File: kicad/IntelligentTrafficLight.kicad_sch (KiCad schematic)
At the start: 62 parts, among them J1 Conn_01x03_Pin, J2 Conn_01x10_Socket, J3 USB-C Receptacle, J4 Conn_01x07_Socket, J5 Conn_01x07_Socket, SW1 Pushbutton, SW2 Pushbutton, U1 ESP32-C3-MINI-1-H4X, U2 PCA9685PW, U3 TLV76133DCY, U4 MAX40200AUK

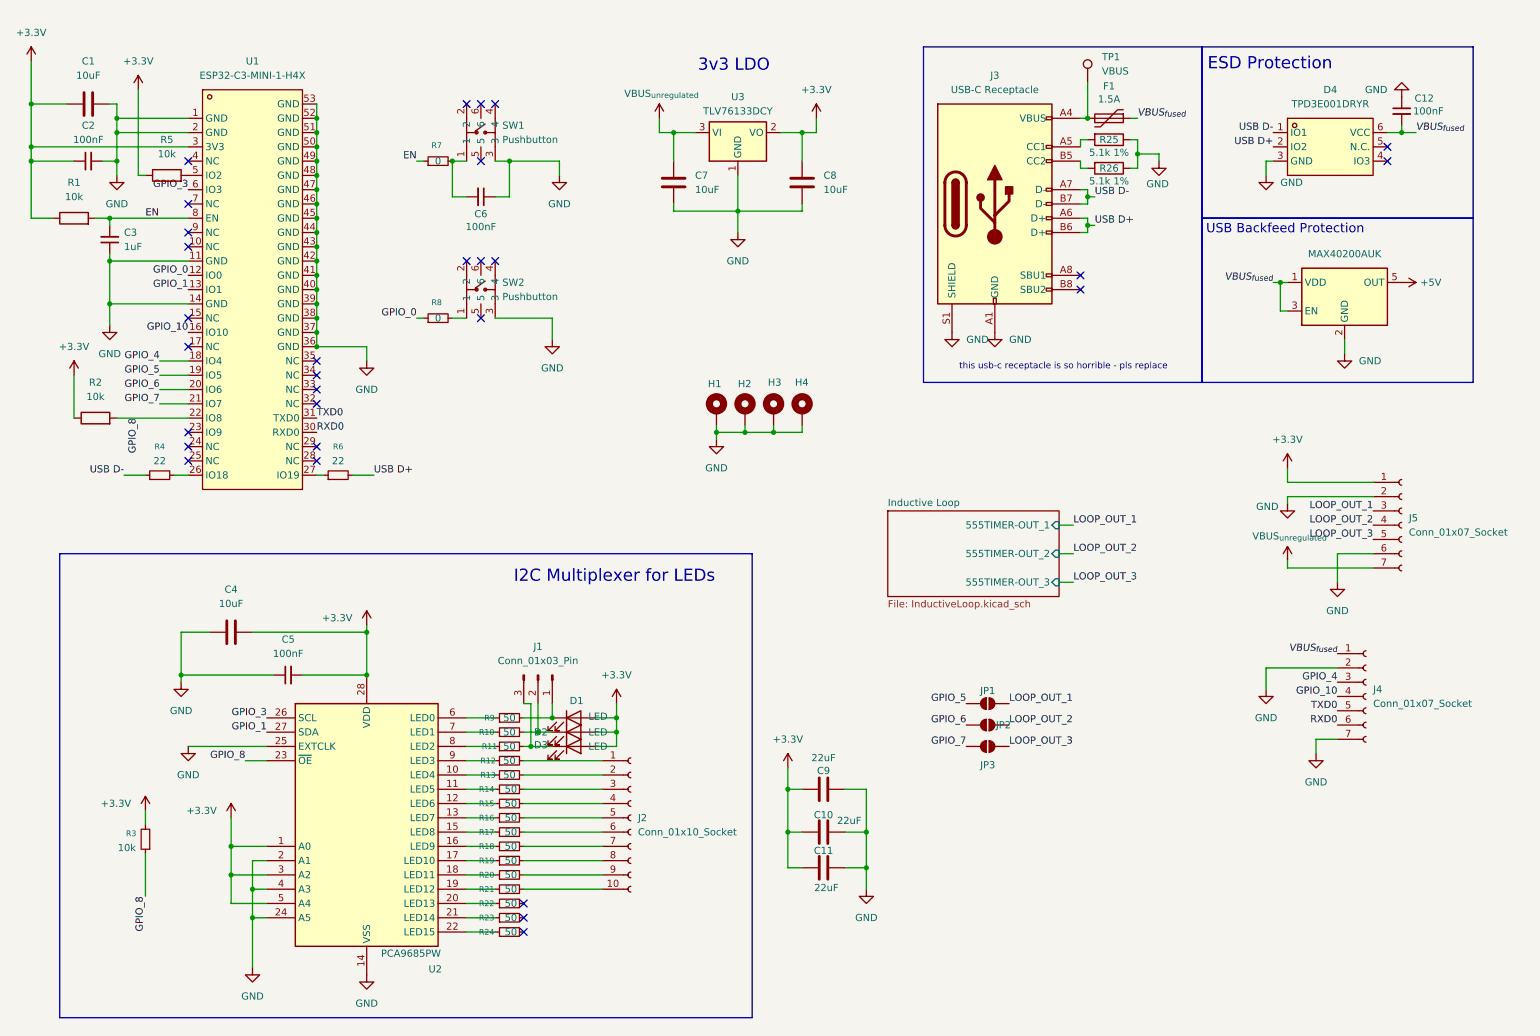
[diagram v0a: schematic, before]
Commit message: small pcb change
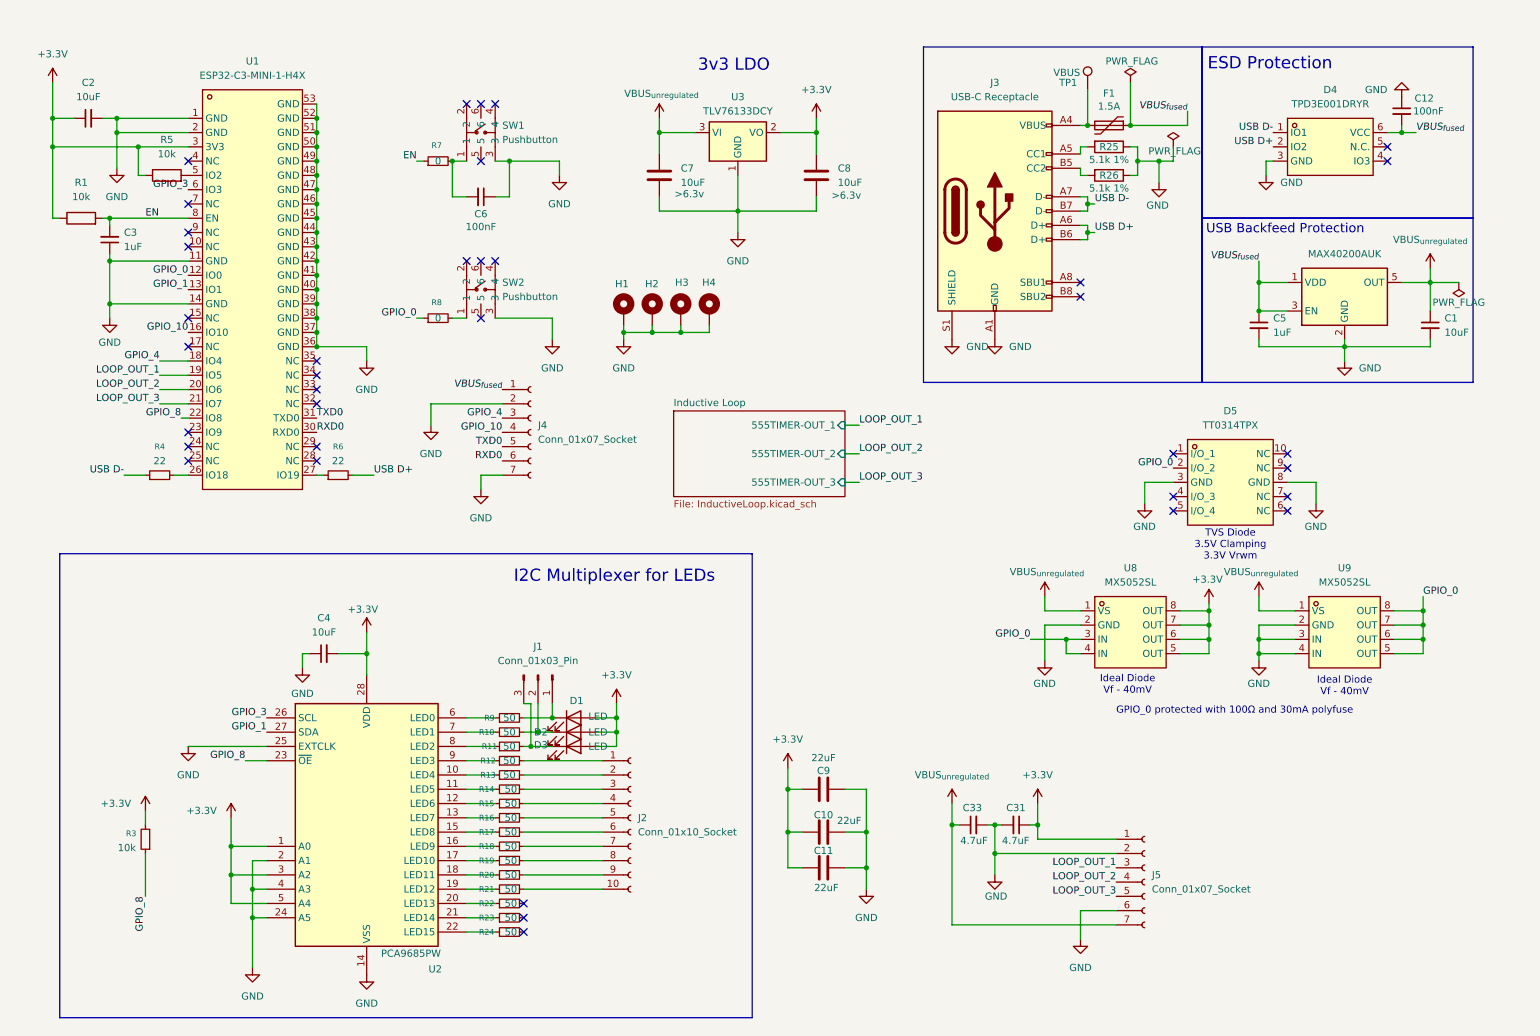
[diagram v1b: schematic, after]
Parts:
- removed C1, C4: 10uF, Capacitor_SMD:C_0402_1005Metric, symbol Device:C
- removed JP1, JP2, JP3: SolderJumper_2_Open, Jumper:SolderJumper-2_P1.3mm_Open_RoundedPad1.0x1.5mm, symbol Jumper:SolderJumper_2_Open
- removed R2: 10k, Resistor_SMD:R_0402_1005Metric, symbol Device:R
- added C1, C4: 10uF, Capacitor_SMD:C_0402_1005Metric, symbol Device:C_Small
- added C31, C33: 4.7uF, Capacitor_SMD:C_0402_1005Metric, symbol Device:C_Small
- added D5: TT0314TPX, easyeda2kicad:DFN2510-10_L2.5-W1.0-P0.50-BL, symbol EASYEDA2KICAD:TT0314TPX
- added U8, U9: MX5052SL, easyeda2kicad:SOP-8_L5.1-W3.9-P1.27-LS6.0-BL, symbol EASYEDA2KICAD:MX5052SL
- C2: value 100nF -> 10uF
- C5: value 100nF -> 1uF
- C7, C8: Voltage Rating (none) -> >6.3v
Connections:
- net +5V is gone; now on net VBUS_{unregulated}: U4.5 (OUT)
- net GPIO_5 is gone; now on net LOOP_OUT_1: U1.19 (IO5)
- net GPIO_6 is gone; now on net LOOP_OUT_2: U1.20 (IO6)
- net GPIO_7 is gone; now on net LOOP_OUT_3: U1.21 (IO7)
- net +3.3V: now also C31.1, C4.2, U8.5 (OUT), U8.6 (OUT), U8.7 (OUT), U8.8 (OUT); no longer C5.2
- net GND: now also C5.2, C1.2, C31.2, C33.2, C4.1, D5.3 (GND), D5.8 (GND), U8.2 (GND), U9.2 (GND), U9.3 (IN), U9.4 (IN); no longer C5.1
- net GPIO_0: now also D5.2 (I/O_2), U8.3 (IN), U8.4 (IN), U9.5 (OUT), U9.6 (OUT), U9.7 (OUT), U9.8 (OUT)
- net VBUS_{fused}: now also C5.1
- net VBUS_{unregulated}: now also C1.1, C33.1, U8.1 (VS), U9.1 (VS)
- no-connect marks 30 -> 37
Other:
- note added: "GPIO_0 protected with 100Ω and 30mA polyfuse"
- note added: "Ideal Diode Vf - 40mV"
- note added: "TVS Diode 3.5V Clamping 3.3V Vrwm"
- note removed: "this usb-c receptacle is so horrible - pls replace"
- moved on the sheet: C7, C8, F1, H1, H2, H3, H4, J3, J4, J5, R1, R25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

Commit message: update!
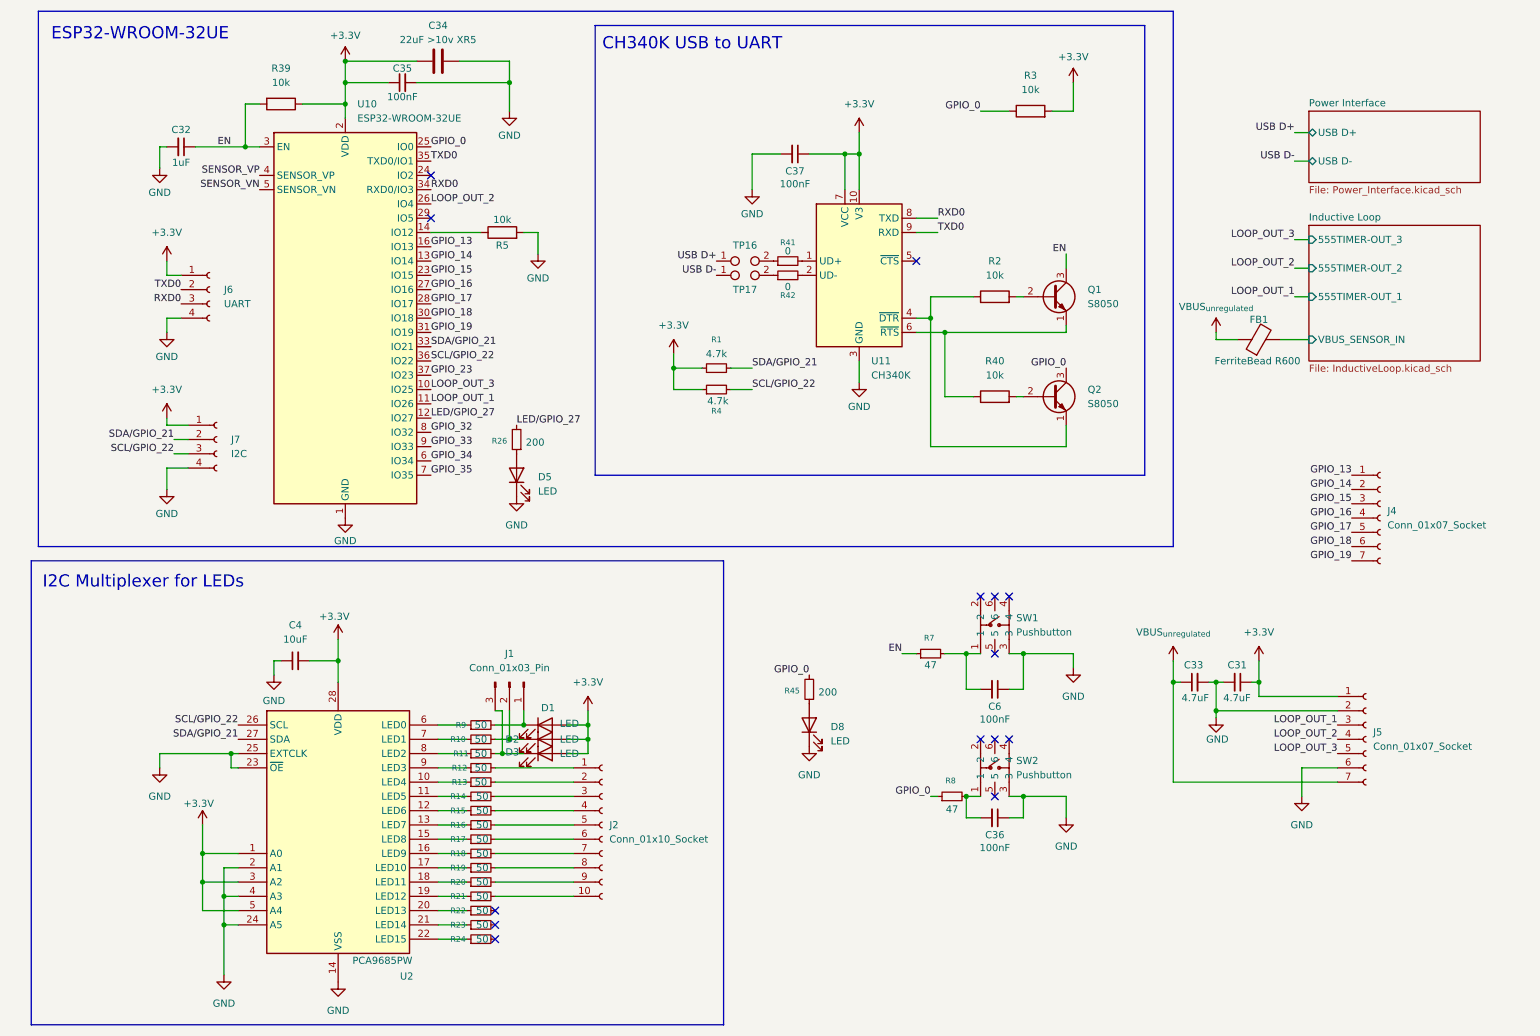
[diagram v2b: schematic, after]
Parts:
- removed C1, C2: 10uF, Capacitor_SMD:C_0402_1005Metric, symbol Device:C_Small
- removed C10, C11, C9: 22uF, Capacitor_SMD:C_0805_2012Metric, symbol Device:C
- removed C12: 100nF, Capacitor_SMD:C_0402_1005Metric, symbol Device:C_Small
- removed C3, C5: 1uF, Capacitor_SMD:C_0402_1005Metric, symbol Device:C_Small
- removed C7, C8: 10uF, Capacitor_SMD:C_0402_1005Metric, symbol Device:C
- removed D4: TPD3E001DRYR, Package_SON:Texas_USON-6_1x1.45mm_P0.5mm_SMD, symbol EasyEDA:TPD3E001DRYR
- removed D5: TT0314TPX, easyeda2kicad:DFN2510-10_L2.5-W1.0-P0.50-BL, symbol EASYEDA2KICAD:TT0314TPX
- removed F1: 1.5A, Fuse:Fuse_1206_3216Metric_Pad1.42x1.75mm_HandSolder, symbol Device:Polyfuse
- removed H1, H2, H3, H4: MountingHole_Pad, MountingHole:MountingHole_3.2mm_M3_Pad, symbol Mechanical:MountingHole_Pad
- removed J3: USB-C Receptacle, Connector_USB:USB_C_Receptacle_G-Switch_GT-USB-7010ASV, symbol Connector:USB_C_Receptacle_USB2.0_16P
- removed R1: 10k, Resistor_SMD:R_0402_1005Metric, symbol Device:R
- removed R25, R26: 5.1k 1%, Resistor_SMD:R_0402_1005Metric, symbol Device:R
- removed R3: 10k, Resistor_SMD:R_0402_1005Metric, symbol Device:R_Small
- removed R6: 22, Resistor_SMD:R_0402_1005Metric, symbol Device:R_Small
- removed TP1: VBUS, Connector_PinSocket_2.54mm:PinSocket_1x01_P2.54mm_Vertical, symbol Connector:TestPoint
- removed U1: ESP32-C3-MINI-1-H4X, EASYEDA2KICAD:WIFIM-SMD_ESP32-C3-MINI-1, symbol EASYEDA2KICAD:ESP32-C3-MINI-1-H4X
- removed U3: TLV76133DCY, Package_TO_SOT_SMD:SOT-223-3_TabPin2, symbol Regulator_Linear:TLV76133DCY
- removed U4: MAX40200AUK, Package_TO_SOT_SMD:SOT-23-5, symbol Analog_Switch:MAX40200AUK
- removed U8, U9: MX5052SL, easyeda2kicad:SOP-8_L5.1-W3.9-P1.27-LS6.0-BL, symbol EASYEDA2KICAD:MX5052SL
- added C32: 1uF, Capacitor_SMD:C_0402_1005Metric, symbol Device:C_Small
- added C34: 22uF >10v XR5, Capacitor_SMD:C_0805_2012Metric, symbol Device:C
- added C35, C36, C37: 100nF, Capacitor_SMD:C_0402_1005Metric, symbol Device:C_Small
- added D5, D8: LED, LED_THT:LED_D5.0mm, symbol Device:LED
- added FB1: FerriteBead R600, Inductor_SMD:L_0603_1608Metric, symbol Device:FerriteBead
- added J6: UART, symbol Connector:Conn_01x04_Socket
- added J7: I2C, symbol Connector:Conn_01x04_Socket
- added Q1, Q2: S8050, Package_TO_SOT_THT:TO-92_Inline, symbol Transistor_BJT:S8050
- added R1: 4.7k, Resistor_SMD:R_0402_1005Metric, symbol Device:R_Small
- added R2, R3, R39, R40: 10k, Resistor_SMD:R_0402_1005Metric, symbol Device:R
- added R26, R45: 200, Resistor_SMD:R_0402_1005Metric, symbol Device:R_Small
- added R41, R42: 0, Resistor_SMD:R_0603_1608Metric, symbol Device:R_Small
- added TP16, TP17: TestPoint_2Pole, TestPoint:TestPoint_Bridge_Pitch3.81mm_Drill1.3mm, symbol Connector:TestPoint_2Pole
- added U10: ESP32-WROOM-32UE, RF_Module:ESP32-WROOM-32UE, symbol RF_Module:ESP32-WROOM-32UE
- added U11: CH340K, Package_SO:SSOP-10-1EP_3.9x4.9mm_P1mm_EP2.1x3.3mm, symbol Interface_USB:CH340K
- R4: value 22 -> 4.7k
- R7, R8: value 0 -> 47
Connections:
- net GPIO_3 is gone; now on net SCL/GPIO_22: U2.26 (SCL)
- net GPIO_8 is gone; now on net GND: U2.23 (~{OE})
- net +3.3V: now also R4.1, C34.1, C35.1, C37.1, J6.1 (Pin_1), J7.1 (Pin_1), R1.1, R3.2, R39.1, U10.2 (VDD), U11.10 (V3), U11.7 (VCC); no longer R5.1
- net EN: now also C32.1, Q1.3 (C), R39.2, U10.3 (EN)
- net GND: now also R5.2, C32.2, C34.2, C35.2, C36.1, C37.2, D5.1 (K), D8.1 (K), J6.4 (Pin_4), J7.4 (Pin_4), U10.1 (GND), U10.15 (GND), U10.38 (GND), U10.39 (GND), U11.11 (GND), U11.3 (GND); no longer J4.2 (Pin_2), J4.7 (Pin_7)
- net GPIO_0: now also Q2.3 (C), R3.1, R45.2, U10.25 (IO0)
- net LOOP_OUT_1: now also U10.11 (IO26)
- net LOOP_OUT_2: now also U10.26 (IO4)
- net LOOP_OUT_3: now also U10.10 (IO25)
- net RXD0: now also J6.3 (Pin_3), U10.34 (RXD0/IO3), U11.8 (TXD); no longer J4.6 (Pin_6)
- net TXD0: now also J6.2 (Pin_2), U10.35 (TXD0/IO1), U11.9 (RXD); no longer J4.5 (Pin_5)
- net USB D+: now also TP16.1
- net USB D-: now also TP17.1; no longer R4.1
- net VBUS_{unregulated}: now also FB1.1
- net at R8.2, SW2.1: now also C36.2
- net SCL/GPIO_22: now reaches R4.2
- net SCL/GPIO_22: now also J7.3 (Pin_3), U10.36 (IO22)
- net GPIO_1 renamed SDA/GPIO_21
- net SDA/GPIO_21: now also J7.2 (Pin_2), R1.2, U10.33 (IO21)
- net GPIO_10 renamed GPIO_16
- net GPIO_16: now also U10.27 (IO16)
- net GPIO_4 renamed GPIO_15
- net GPIO_15: now also U10.23 (IO15)
- net VBUS_{fused} renamed GPIO_13
- net GPIO_13: now also U10.16 (IO13)
- new net: Q2.1 (E), R2.1, U11.4 (~{DTR})
- new net: Q2.2 (B), R40.2
- new net: Q1.1 (E), R40.1, U11.6 (~{RTS})
- new net: R42.1, TP17.2
- new net: R42.2, U11.2 (UD-)
- new net: Q1.2 (B), R2.2
- new net: R5.1, U10.14 (IO12)
- new net: D8.2 (A), R45.1
- new net: D5.2 (A), R26.1
- new net: R41.1, TP16.2
- new net: R41.2, U11.1 (UD+)
- new net GPIO_14: J4.2 (Pin_2), U10.13 (IO14)
- new net GPIO_17: J4.5 (Pin_5), U10.28 (IO17)
- new net GPIO_18: J4.6 (Pin_6), U10.30 (IO18)
- new net GPIO_19: J4.7 (Pin_7), U10.31 (IO19)
- new net GPIO_23: U10.37 (IO23)
- new net GPIO_32: U10.8 (IO32)
- new net GPIO_33: U10.9 (IO33)
- new net GPIO_34: U10.6 (IO34)
- new net GPIO_35: U10.7 (IO35)
- new net Inductive Loop/VBUS_SENSOR_IN: FB1.2
- new net LED/GPIO_27: R26.2, U10.12 (IO27)
- new net SENSOR_VN: U10.5 (SENSOR_VN)
- new net SENSOR_VP: U10.4 (SENSOR_VP)
- no-connect marks 37 -> 14
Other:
- added sheet Power Interface (Power_Interface.kicad_sch)
- sheet Inductive Loop ports: added VBUS_SENSOR_IN; removed none
- note added: "CH340K USB to UART"
- note added: "ESP32-WROOM-32UE"
- note removed: "3v3 LDO"
- note removed: "ESD Protection"
- note removed: "GPIO_0 protected with 100Ω and 30mA polyfuse"
- note removed: "Ideal Diode Vf - 40mV"
- note removed: "TVS Diode 3.5V Clamping 3.3V Vrwm"
- note removed: "USB Backfeed Protection"
- moved on the sheet: C31, C33, C4, C6, D1, D2, D3, J1, J2, J4, J5, R10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
